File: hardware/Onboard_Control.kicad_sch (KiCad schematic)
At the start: 5 parts, among them SW1 CK_KMS2xxG, SW2 CK_KMS2xxG, SW3 CK_KMS2xxG, SW4 CK_KMS2xxG, SW5 CK_KMS2xxG

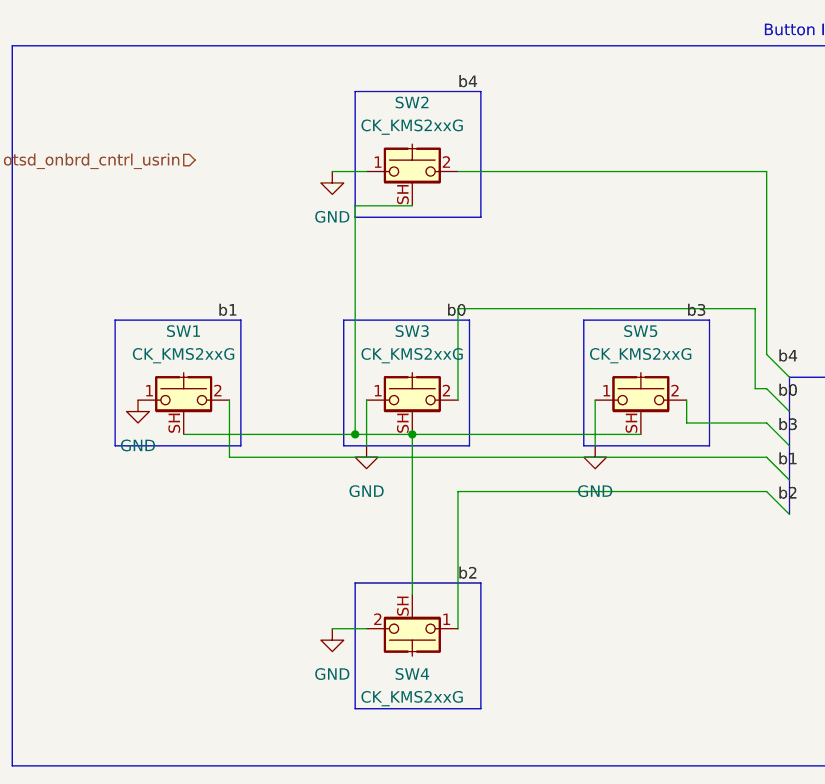
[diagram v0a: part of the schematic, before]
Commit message: Revert "chore(schematic): Update references"
This reverts commit 2cda2d22061e90f93ddb38c43ecf32892cd7b43c.
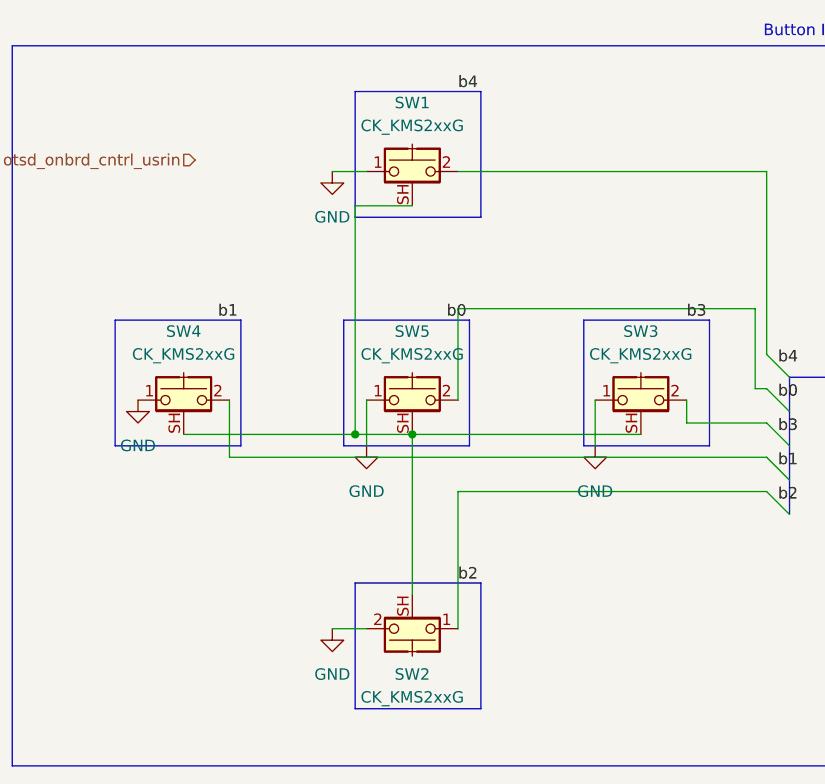
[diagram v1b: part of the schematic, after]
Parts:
- renumbered SW2 to SW1, SW4 to SW2, SW5 to SW3, SW1 to SW4, SW3 to SW5
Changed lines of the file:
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@@
 		(dnp no)
 		(fields_autoplaced yes)
-		(property "Reference" "#PWR018"
+		(property "Reference" "#PWR05"
 			(at 59.69 114.3 0)
 			(effects
@@
 			(project "gpu-external-power-supply"
 				(path "/d5303413-7068-41ba-88e3-39dfa38d31b7/5068f4fb-295f-4c02-a1ca-8a4133aa46e7"
-					(reference "#PWR018")
+					(reference "#PWR05")
 					(unit 1)
 				)
@@
 		(dnp no)
 		(fields_autoplaced yes)
-		(property "Reference" "SW1"
+		(property "Reference" "SW4"
 			(at 39.37 95.25 0)
 			(effects
@@
 			(project "gpu-external-power-supply"
 				(path "/d5303413-7068-41ba-88e3-39dfa38d31b7/5068f4fb-295f-4c02-a1ca-8a4133aa46e7"
-					(reference "SW1")
+					(reference "SW4")
 					(unit 1)
 				)
@@
 		(dnp no)
 		(fields_autoplaced yes)
-		(property "Reference" "#PWR015"
+		(property "Reference" "#PWR04"
 			(at 34.29 109.22 0)
 			(effects
@@
 			(project "gpu-external-power-supply"
 				(path "/d5303413-7068-41ba-88e3-39dfa38d31b7/5068f4fb-295f-4c02-a1ca-8a4133aa46e7"
-					(reference "#PWR015")
+					(reference "#PWR04")
 					(unit 1)
 				)
@@
 		(dnp no)
 		(fields_autoplaced yes)
-		(property "Reference" "SW4"
+		(property "Reference" "SW2"
 			(at 64.77 133.35 0)
 			(effects
@@
 			(project "gpu-external-power-supply"
 				(path "/d5303413-7068-41ba-88e3-39dfa38d31b7/5068f4fb-295f-4c02-a1ca-8a4133aa46e7"
-					(reference "SW4")
+					(reference "SW2")
 					(unit 1)
 				)
@@
 		(dnp no)
 		(fields_autoplaced yes)
-		(property "Reference" "SW5"
+		(property "Reference" "SW3"
 			(at 90.17 95.25 0)
 			(effects
@@
 			(project "gpu-external-power-supply"
 				(path "/d5303413-7068-41ba-88e3-39dfa38d31b7/5068f4fb-295f-4c02-a1ca-8a4133aa46e7"
-					(reference "SW5")
+					(reference "SW3")
 					(unit 1)
 				)
@@
 		(dnp no)
 		(fields_autoplaced yes)
-		(property "Reference" "SW2"
+		(property "Reference" "SW1"
 			(at 64.77 69.85 0)
 			(effects
@@
 			(project ""
 				(path "/d5303413-7068-41ba-88e3-39dfa38d31b7/5068f4fb-295f-4c02-a1ca-8a4133aa46e7"
-					(reference "SW2")
+					(reference "SW1")
 					(unit 1)
 				)
@@
 		(dnp no)
 		(fields_autoplaced yes)
-		(property "Reference" "#PWR019"
+		(property "Reference" "#PWR06"
 			(at 85.09 114.3 0)
 			(effects
@@
 			(project "gpu-external-power-supply"
 				(path "/d5303413-7068-41ba-88e3-39dfa38d31b7/5068f4fb-295f-4c02-a1ca-8a4133aa46e7"
-					(reference "#PWR019")
+					(reference "#PWR06")
 					(unit 1)
 				)
@@
 		(dnp no)
 		(fields_autoplaced yes)
-		(property "Reference" "SW3"
+		(property "Reference" "SW5"
 			(at 64.77 95.25 0)
 			(effects
@@
 			(project "gpu-external-power-supply"
 				(path "/d5303413-7068-41ba-88e3-39dfa38d31b7/5068f4fb-295f-4c02-a1ca-8a4133aa46e7"
-					(reference "SW3")
+					(reference "SW5")
 					(unit 1)
 				)
@@
 		(dnp no)
 		(fields_autoplaced yes)
-		(property "Reference" "#PWR017"
+		(property "Reference" "#PWR07"
 			(at 55.88 134.62 0)
 			(effects
@@
 			(project "gpu-external-power-supply"
 				(path "/d5303413-7068-41ba-88e3-39dfa38d31b7/5068f4fb-295f-4c02-a1ca-8a4133aa46e7"
-					(reference "#PWR017")
+					(reference "#PWR07")
 					(unit 1)
 				)
@@
 		(dnp no)
 		(fields_autoplaced yes)
-		(property "Reference" "#PWR016"
+		(property "Reference" "#PWR03"
 			(at 55.88 83.82 0)
 			(effects
@@
 			(project "gpu-external-power-supply"
 				(path "/d5303413-7068-41ba-88e3-39dfa38d31b7/5068f4fb-295f-4c02-a1ca-8a4133aa46e7"
-					(reference "#PWR016")
-					(unit 1)
-				)
+					(reference "#PWR03")
+					(unit 1)
+				)

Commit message: chore(schematic): Update references
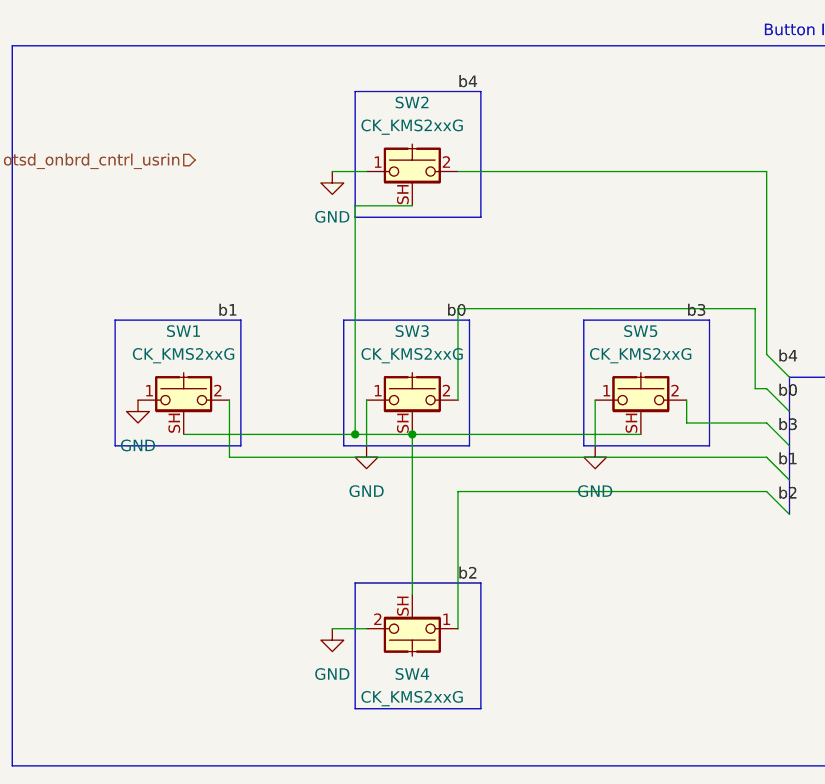
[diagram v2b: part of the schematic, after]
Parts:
- renumbered SW4 to SW1, SW1 to SW2, SW5 to SW3, SW2 to SW4, SW3 to SW5
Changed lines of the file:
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@@
 		(dnp no)
 		(fields_autoplaced yes)
-		(property "Reference" "#PWR05"
+		(property "Reference" "#PWR018"
 			(at 59.69 114.3 0)
 			(effects
@@
 			(project "gpu-external-power-supply"
 				(path "/d5303413-7068-41ba-88e3-39dfa38d31b7/5068f4fb-295f-4c02-a1ca-8a4133aa46e7"
-					(reference "#PWR05")
+					(reference "#PWR018")
 					(unit 1)
 				)
@@
 		(dnp no)
 		(fields_autoplaced yes)
-		(property "Reference" "SW4"
+		(property "Reference" "SW1"
 			(at 39.37 95.25 0)
 			(effects
@@
 			(project "gpu-external-power-supply"
 				(path "/d5303413-7068-41ba-88e3-39dfa38d31b7/5068f4fb-295f-4c02-a1ca-8a4133aa46e7"
-					(reference "SW4")
+					(reference "SW1")
 					(unit 1)
 				)
@@
 		(dnp no)
 		(fields_autoplaced yes)
-		(property "Reference" "#PWR04"
+		(property "Reference" "#PWR015"
 			(at 34.29 109.22 0)
 			(effects
@@
 			(project "gpu-external-power-supply"
 				(path "/d5303413-7068-41ba-88e3-39dfa38d31b7/5068f4fb-295f-4c02-a1ca-8a4133aa46e7"
-					(reference "#PWR04")
+					(reference "#PWR015")
 					(unit 1)
 				)
@@
 		(dnp no)
 		(fields_autoplaced yes)
-		(property "Reference" "SW2"
+		(property "Reference" "SW4"
 			(at 64.77 133.35 0)
 			(effects
@@
 			(project "gpu-external-power-supply"
 				(path "/d5303413-7068-41ba-88e3-39dfa38d31b7/5068f4fb-295f-4c02-a1ca-8a4133aa46e7"
-					(reference "SW2")
+					(reference "SW4")
 					(unit 1)
 				)
@@
 		(dnp no)
 		(fields_autoplaced yes)
-		(property "Reference" "SW3"
+		(property "Reference" "SW5"
 			(at 90.17 95.25 0)
 			(effects
@@
 			(project "gpu-external-power-supply"
 				(path "/d5303413-7068-41ba-88e3-39dfa38d31b7/5068f4fb-295f-4c02-a1ca-8a4133aa46e7"
-					(reference "SW3")
+					(reference "SW5")
 					(unit 1)
 				)
@@
 		(dnp no)
 		(fields_autoplaced yes)
-		(property "Reference" "SW1"
+		(property "Reference" "SW2"
 			(at 64.77 69.85 0)
 			(effects
@@
 			(project ""
 				(path "/d5303413-7068-41ba-88e3-39dfa38d31b7/5068f4fb-295f-4c02-a1ca-8a4133aa46e7"
-					(reference "SW1")
+					(reference "SW2")
 					(unit 1)
 				)
@@
 		(dnp no)
 		(fields_autoplaced yes)
-		(property "Reference" "#PWR06"
+		(property "Reference" "#PWR019"
 			(at 85.09 114.3 0)
 			(effects
@@
 			(project "gpu-external-power-supply"
 				(path "/d5303413-7068-41ba-88e3-39dfa38d31b7/5068f4fb-295f-4c02-a1ca-8a4133aa46e7"
-					(reference "#PWR06")
+					(reference "#PWR019")
 					(unit 1)
 				)
@@
 		(dnp no)
 		(fields_autoplaced yes)
-		(property "Reference" "SW5"
+		(property "Reference" "SW3"
 			(at 64.77 95.25 0)
 			(effects
@@
 			(project "gpu-external-power-supply"
 				(path "/d5303413-7068-41ba-88e3-39dfa38d31b7/5068f4fb-295f-4c02-a1ca-8a4133aa46e7"
-					(reference "SW5")
+					(reference "SW3")
 					(unit 1)
 				)
@@
 		(dnp no)
 		(fields_autoplaced yes)
-		(property "Reference" "#PWR07"
+		(property "Reference" "#PWR017"
 			(at 55.88 134.62 0)
 			(effects
@@
 			(project "gpu-external-power-supply"
 				(path "/d5303413-7068-41ba-88e3-39dfa38d31b7/5068f4fb-295f-4c02-a1ca-8a4133aa46e7"
-					(reference "#PWR07")
+					(reference "#PWR017")
 					(unit 1)
 				)
@@
 		(dnp no)
 		(fields_autoplaced yes)
-		(property "Reference" "#PWR03"
+		(property "Reference" "#PWR016"
 			(at 55.88 83.82 0)
 			(effects
@@
 			(project "gpu-external-power-supply"
 				(path "/d5303413-7068-41ba-88e3-39dfa38d31b7/5068f4fb-295f-4c02-a1ca-8a4133aa46e7"
-					(reference "#PWR03")
-					(unit 1)
-				)
+					(reference "#PWR016")
+					(unit 1)
+				)
